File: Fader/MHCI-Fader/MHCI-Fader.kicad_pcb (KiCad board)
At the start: 2 copper layers, 107.5 x 20 mm, 31 parts, among them J1 Conn_01x06, SW1 SW_Push_LED, U3 SRV05-4, U4 TXB0102DCU, U5 TJA1051T-3

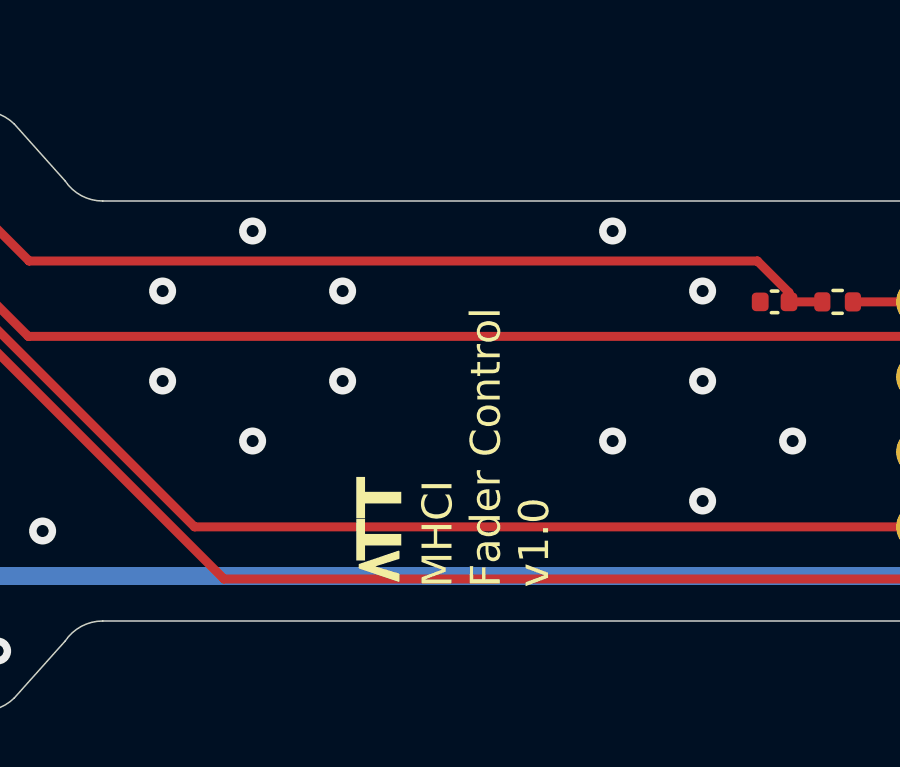
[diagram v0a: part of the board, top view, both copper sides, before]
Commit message: MHCI Production Read
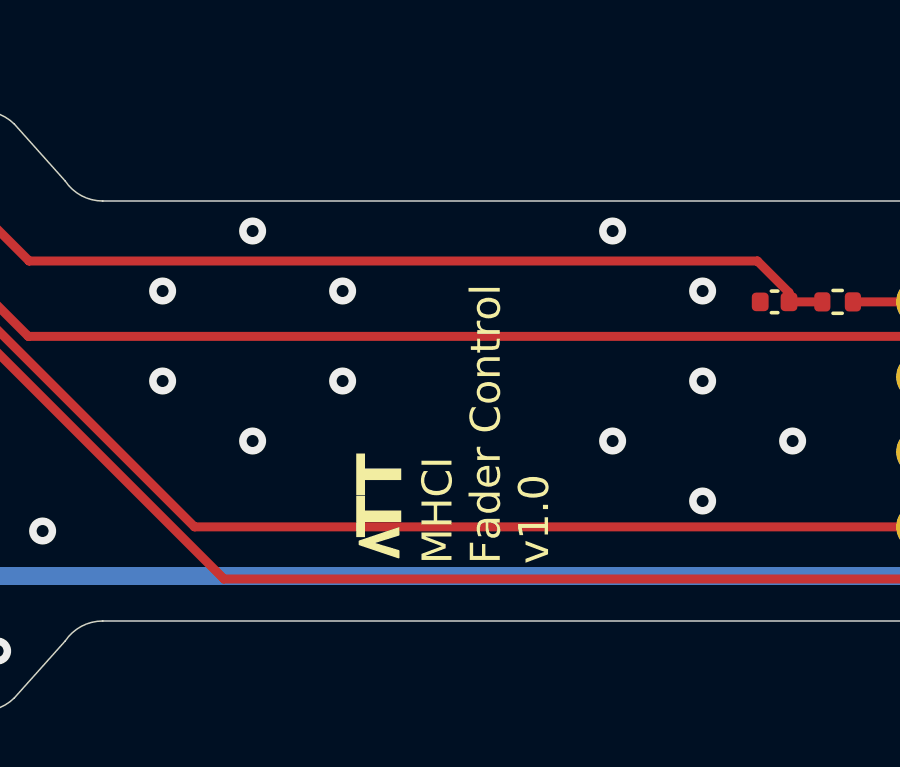
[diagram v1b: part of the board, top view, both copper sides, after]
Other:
- board text removed: "TOOLING HOLES MOUNTING HOLES"
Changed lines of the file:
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@@
 	(gr_poly
 		(pts
-			(xy 138.871244 106.68) (xy 137.561246 107.120002) (xy 137.561245 107.230002) (xy 138.871244 107.67)
-			(xy 138.871246 107.440002) (xy 138.001247 107.180002) (xy 138.871244 106.910002)
+			(xy 138.869997 105.899998) (xy 137.559999 106.34) (xy 137.559998 106.45) (xy 138.869997 106.889998)
+			(xy 138.869999 106.66) (xy 138 106.4) (xy 138.869997 106.13)
 		)
 		(stroke
@@
 	)
 	(gr_text "MHCI\nFader Control\nv1.0"
-		(at 143.971244 107.880001 90)
+		(at 143.969997 107.099999 90)
 		(layer "F.SilkS")
 		(effects
@@
 	)
 	(gr_text "TT"
-		(at 138.261247 105.590002 90)
+		(at 138.26 104.81 90)
 		(layer "F.SilkS")
 		(effects
@@
 			(polygon
 				(pts
-					(xy 138.883747 106.236268) (xy 137.771098 106.236268) (xy 137.771098 106.590908) (xy 137.570697 106.590908)
-					(xy 137.570697 105.634698) (xy 137.771098 105.634698) (xy 137.771098 106.008389) (xy 138.883747 106.008389)
+					(xy 138.8825 105.456266) (xy 137.769851 105.456266) (xy 137.769851 105.810906) (xy 137.56945 105.810906)
+					(xy 137.56945 104.854696) (xy 137.769851 104.854696) (xy 137.769851 105.228387) (xy 138.8825 105.228387)
 				)
 			)
 			(polygon
 				(pts
-					(xy 138.883747 105.187001) (xy 137.771098 105.187001) (xy 137.771098 105.541641) (xy 137.570697 105.541641)
-					(xy 137.570697 104.58543) (xy 137.771098 104.58543) (xy 137.771098 104.959122) (xy 138.883747 104.959122)
+					(xy 138.8825 104.406999) (xy 137.769851 104.406999) (xy 137.769851 104.761639) (xy 137.56945 104.761639)
+					(xy 137.56945 103.805428) (xy 137.769851 103.805428) (xy 137.769851 104.17912) (xy 138.8825 104.17912)
 				)
 			)
@@
 		)
 	)
-	(gr_text "TOOLING HOLES\nMOUNTING HOLES"
-		(at 102 123 0)
-		(layer "Dwgs.User")
-		(effects
-			(font
-				(size 3 3)
-				(thickness 0.6)
-				(bold yes)
-			)
-			(justify left bottom)
-		)
-	)
